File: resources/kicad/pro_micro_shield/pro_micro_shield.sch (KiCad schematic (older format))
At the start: 19 parts, among them U0 ProMicro

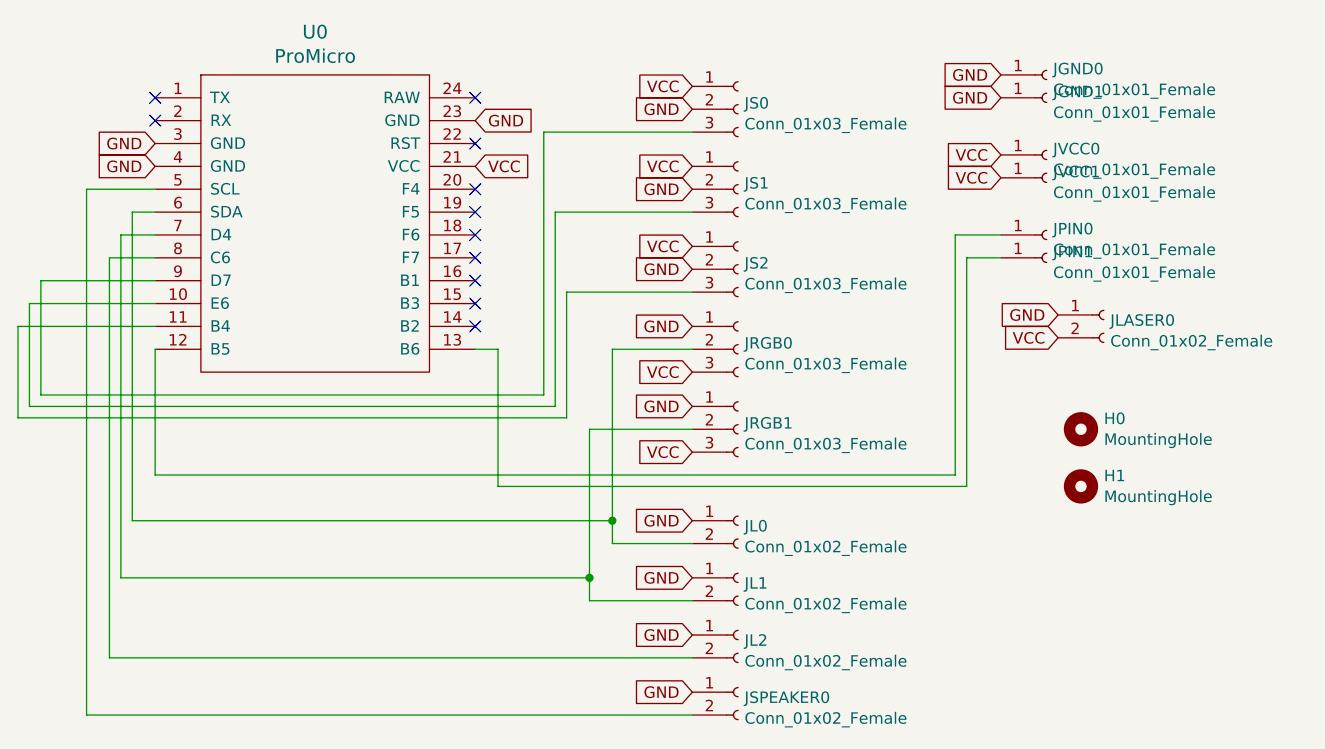
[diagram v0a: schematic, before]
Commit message: shield pcb revision 2
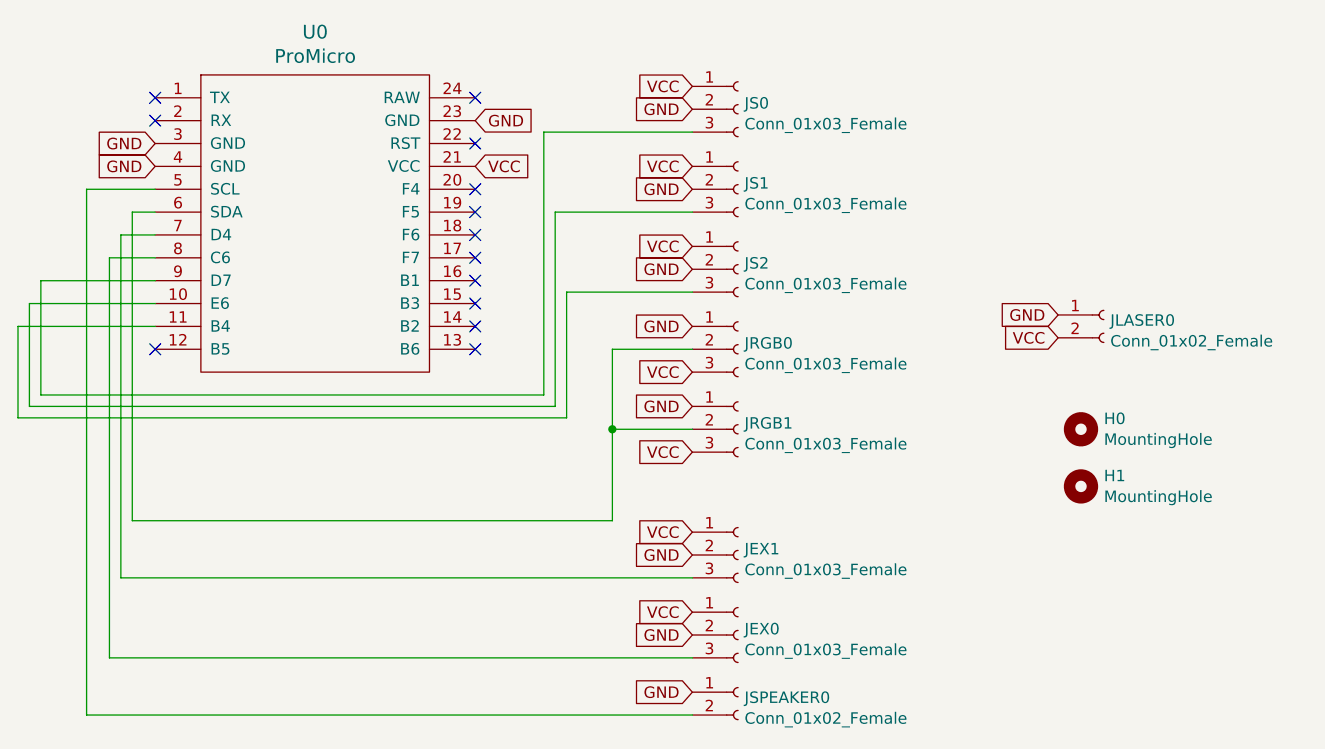
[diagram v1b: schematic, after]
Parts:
- removed JGND0, JGND1, JPIN0, JPIN1, JVCC0, JVCC1: Conn_01x01_Female, Connector_Wire:SolderWirePad_1x01_Drill1mm, symbol Connector:Conn_01x01_Female
- removed JL0, JL1, JL2: Conn_01x02_Female, Connector_Wire:SolderWirePad_1x02_P3.81mm_Drill1mm, symbol Connector:Conn_01x02_Female
- added JEX0, JEX1: Conn_01x03_Female, Connector_Wire:SolderWirePad_1x03_P3.175mm_Drill1mm, symbol Connector:Conn_01x03_Female
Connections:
- net GND: now also JEX0.2 (Pin_2), JEX1.2 (Pin_2)
- net VCC: now also JEX0.1 (Pin_1), JEX1.1 (Pin_1)
- net at JRGB0.2 (Pin_2), U0.6 (SDA): now also JRGB1.2 (Pin_2)
- net at U0.7 (D4): now also JEX1.3 (Pin_3); no longer JRGB1.2 (Pin_2)
- net at U0.8 (C6): now also JEX0.3 (Pin_3)
- no-connect marks 11 -> 13
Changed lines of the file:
@@
-	1    0    0    -1
-$EndComp
-$Comp
-L Connector:Conn_01x02_Female JL0
-U 1 1 5E63EBB8
-P 5850 4950
-F 0 "JL0" H 5878 4926 50  0000 L CNN
-F 1 "Conn_01x02_Female" H 5878 4835 50  0000 L CNN
-F 2 "Connector_Wire:SolderWirePad_1x02_P3.81mm_Drill1mm" H 5850 4950 50  0001 C CNN
-F 3 "~" H 5850 4950 50  0001 C CNN
-	1    5850 4950
-	1    0    0    -1
-$EndComp
-$Comp
-L Connector:Conn_01x02_Female JL1
-U 1 1 5E63F977
-P 5850 5200
-F 0 "JL1" H 5878 5176 50  0000 L CNN
-F 1 "Conn_01x02_Female" H 5878 5085 50  0000 L CNN
-F 2 "Connector_Wire:SolderWirePad_1x02_P3.81mm_Drill1mm" H 5850 5200 50  0001 C CNN
-F 3 "~" H 5850 5200 50  0001 C CNN
-	1    5850 5200
-	1    0    0    -1
-$EndComp
-$Comp
-L Connector:Conn_01x02_Female JL2
-U 1 1 5E64015B
-P 5850 5450
-F 0 "JL2" H 5878 5426 50  0000 L CNN
-F 1 "Conn_01x02_Female" H 5878 5335 50  0000 L CNN
-F 2 "Connector_Wire:SolderWirePad_1x02_P3.81mm_Drill1mm" H 5850 5450 50  0001 C CNN
-F 3 "~" H 5850 5450 50  0001 C CNN
-	1    5850 5450
-	1    0    0    -1
-$EndComp
-$Comp
-L Connector:Conn_01x02_Female JSPEAKER0
-U 1 1 5E640A6C
-P 5850 5700
-F 0 "JSPEAKER0" H 5878 5676 50  0000 L CNN
-F 1 "Conn_01x02_Female" H 5878 5585 50  0000 L CNN
-F 2 "Connector_Wire:SolderWirePad_1x02_P3.81mm_Drill1mm" H 5850 5700 50  0001 C CNN
-F 3 "~" H 5850 5700 50  0001 C CNN
-	1    5850 5700
 	1    0    0    -1
 $EndComp
@@
 Text GLabel 5650 4650 0    50   Input ~ 0
 VCC
-Text GLabel 5650 4950 0    50   Input ~ 0
-GND
-Text GLabel 5650 5200 0    50   Input ~ 0
-GND
-Text GLabel 5650 5450 0    50   Input ~ 0
-GND
 Text GLabel 5650 5700 0    50   Input ~ 0
 GND
@@
 	3000 3500 3300 3500
 Wire Wire Line
-	5650 5050 5300 5050
-Wire Wire Line
 	3200 4950 3200 3600
 Wire Wire Line
 	3200 3600 3300 3600
 Wire Wire Line
-	5650 5300 5200 5300
-Wire Wire Line
 	3150 5200 3150 3700
 Wire Wire Line
 	3150 3700 3300 3700
-Wire Wire Line
-	5650 5550 3100 5550
 Wire Wire Line
 	3100 3800 3300 3800
@@
 	5650 4200 5300 4200
 Wire Wire Line
-	5300 4200 5300 4950
-Wire Wire Line
 	5300 4950 3200 4950
-Wire Wire Line
-	5650 4550 5200 4550
-Wire Wire Line
-	5200 4550 5200 5200
-Wire Wire Line
-	5200 5200 3150 5200
-Text GLabel 7000 3000 0    50   Input ~ 0
-GND
-Text GLabel 7000 3100 0    50   Input ~ 0
-GND
-Text GLabel 7000 3350 0    50   Input ~ 0
-VCC
-Text GLabel 7000 3450 0    50   Input ~ 0
-VCC
-Wire Wire Line
-	7000 3700 6800 3700
-Wire Wire Line
-	6800 4750 3300 4750
-Wire Wire Line
-	3300 4750 3300 4200
-Wire Wire Line
-	7000 3800 6850 3800
-Wire Wire Line
-	6850 3800 6850 4800
-Wire Wire Line
-	6850 4800 4800 4800
-Wire Wire Line
-	4800 4800 4800 4200
-Wire Wire Line
-	4800 4200 4700 4200
 NoConn ~ 4700 3100
 NoConn ~ 4700 3300
@@
 NoConn ~ 3300 3200
 Wire Wire Line
-	5300 5050 5300 4950
-Connection ~ 5300 4950
-Wire Wire Line
-	5200 5300 5200 5200
-Connection ~ 5200 5200
-Wire Wire Line
 	3100 3800 3100 5550
 Wire Wire Line
 	3000 3500 3000 5800
-$Comp
-L Connector:Conn_01x01_Female JPIN0
-U 1 1 5E66D93E
-P 7200 3700
-F 0 "JPIN0" H 7228 3726 50  0000 L CNN
-F 1 "Conn_01x01_Female" H 7228 3635 50  0000 L CNN
-F 2 "Connector_Wire:SolderWirePad_1x01_Drill1mm" H 7200 3700 50  0001 C CNN
-F 3 "~" H 7200 3700 50  0001 C CNN
-	1    7200 3700
-	1    0    0    -1
-$EndComp
-Wire Wire Line
-	6800 3700 6800 4750
-$Comp
-L Connector:Conn_01x01_Female JPIN1
-U 1 1 5E66E582
-P 7200 3800
-F 0 "JPIN1" H 7228 3826 50  0000 L CNN
-F 1 "Conn_01x01_Female" H 7228 3735 50  0000 L CNN
-F 2 "Connector_Wire:SolderWirePad_1x01_Drill1mm" H 7200 3800 50  0001 C CNN
-F 3 "~" H 7200 3800 50  0001 C CNN
-	1    7200 3800
-	1    0    0    -1
-$EndComp
 $Comp
 L Mechanical:MountingHole H0
@@
 Text GLabel 7250 4050 0    50   Input ~ 0
 GND
+Wire Wire Line
+	5300 4200 5300 4550
 $Comp
-L Connector:Conn_01x01_Female JGND0
-U 1 1 5E666EF2
-P 7200 3000
-F 0 "JGND0" H 7228 3026 50  0000 L CNN
-F 1 "Conn_01x01_Female" H 7228 2935 50  0000 L CNN
-F 2 "Connector_Wire:SolderWirePad_1x01_Drill1mm" H 7200 3000 50  0001 C CNN
-F 3 "~" H 7200 3000 50  0001 C CNN
-	1    7200 3000
+L Connector:Conn_01x02_Female JSPEAKER0
+U 1 1 5E640A6C
+P 5850 5700
+F 0 "JSPEAKER0" H 5878 5676 50  0000 L CNN
+F 1 "Conn_01x02_Female" H 5878 5585 50  0000 L CNN
+F 2 "Connector_Wire:SolderWirePad_1x02_P3.81mm_Drill1mm" H 5850 5700 50  0001 C CNN
+F 3 "~" H 5850 5700 50  0001 C CNN
+	1    5850 5700
 	1    0    0    -1
 $EndComp
+Wire Wire Line
+	5650 4550 5300 4550
+Connection ~ 5300 4550
+Wire Wire Line
+	5300 4550 5300 4950
 $Comp
-L Connector:Conn_01x01_Female JGND1
-U 1 1 5E667A92
-P 7200 3100
-F 0 "JGND1" H 7228 3126 50  0000 L CNN
-F 1 "Conn_01x01_Female" H 7228 3035 50  0000 L CNN
-F 2 "Connector_Wire:SolderWirePad_1x01_Drill1mm" H 7200 3100 50  0001 C CNN
-F 3 "~" H 7200 3100 50  0001 C CNN
-	1    7200 3100
+L Connector:Conn_01x03_Female JEX0
+U 1 1 5F92E86A
+P 5850 5450
+F 0 "JEX0" H 5878 5476 50  0000 L CNN
+F 1 "Conn_01x03_Female" H 5878 5385 50  0000 L CNN
+F 2 "Connector_Wire:SolderWirePad_1x03_P3.175mm_Drill1mm" H 5850 5450 50  0001 C CNN
+F 3 "~" H 5850 5450 50  0001 C CNN
+	1    5850 5450
 	1    0    0    -1
 $EndComp
+Text GLabel 5650 5350 0    50   Input ~ 0
+VCC
+Text GLabel 5650 5450 0    50   Input ~ 0
+GND
 $Comp
-L Connector:Conn_01x01_Female JVCC0
-U 1 1 5E6684FC
-P 7200 3350
-F 0 "JVCC0" H 7228 3376 50  0000 L CNN
-F 1 "Conn_01x01_Female" H 7228 3285 50  0000 L CNN
-F 2 "Connector_Wire:SolderWirePad_1x01_Drill1mm" H 7200 3350 50  0001 C CNN
-F 3 "~" H 7200 3350 50  0001 C CNN
-	1    7200 3350
+L Connector:Conn_01x03_Female JEX1
+U 1 1 5F930EE7
+P 5850 5100
+F 0 "JEX1" H 5878 5126 50  0000 L CNN
+F 1 "Conn_01x03_Female" H 5878 5035 50  0000 L CNN
+F 2 "Connector_Wire:SolderWirePad_1x03_P3.175mm_Drill1mm" H 5850 5100 50  0001 C CNN
+F 3 "~" H 5850 5100 50  0001 C CNN
+	1    5850 5100
 	1    0    0    -1
 $EndComp
-$Comp
-L Connector:Conn_01x01_Female JVCC1
-U 1 1 5E6689E2
-P 7200 3450
-F 0 "JVCC1" H 7228 3476 50  0000 L CNN
-F 1 "Conn_01x01_Female" H 7228 3385 50  0000 L CNN
-F 2 "Connector_Wire:SolderWirePad_1x01_Drill1mm" H 7200 3450 50  0001 C CNN
-F 3 "~" H 7200 3450 50  0001 C CNN
-	1    7200 3450
-	1    0    0    -1
-$EndComp
+Text GLabel 5650 5000 0    50   Input ~ 0
+VCC
+Text GLabel 5650 5100 0    50   Input ~ 0
+GND
+Wire Wire Line
+	5650 5200 3150 5200
+Wire Wire Line
+	3100 5550 5650 5550
+NoConn ~ 4700 4200
+NoConn ~ 3300 4200
 $EndSCHEMATC
